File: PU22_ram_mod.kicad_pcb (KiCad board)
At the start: 2 copper layers, 39.2 x 94.7 mm, 11 parts, among them J1 MOBO, J2 BA8, J3 BA10

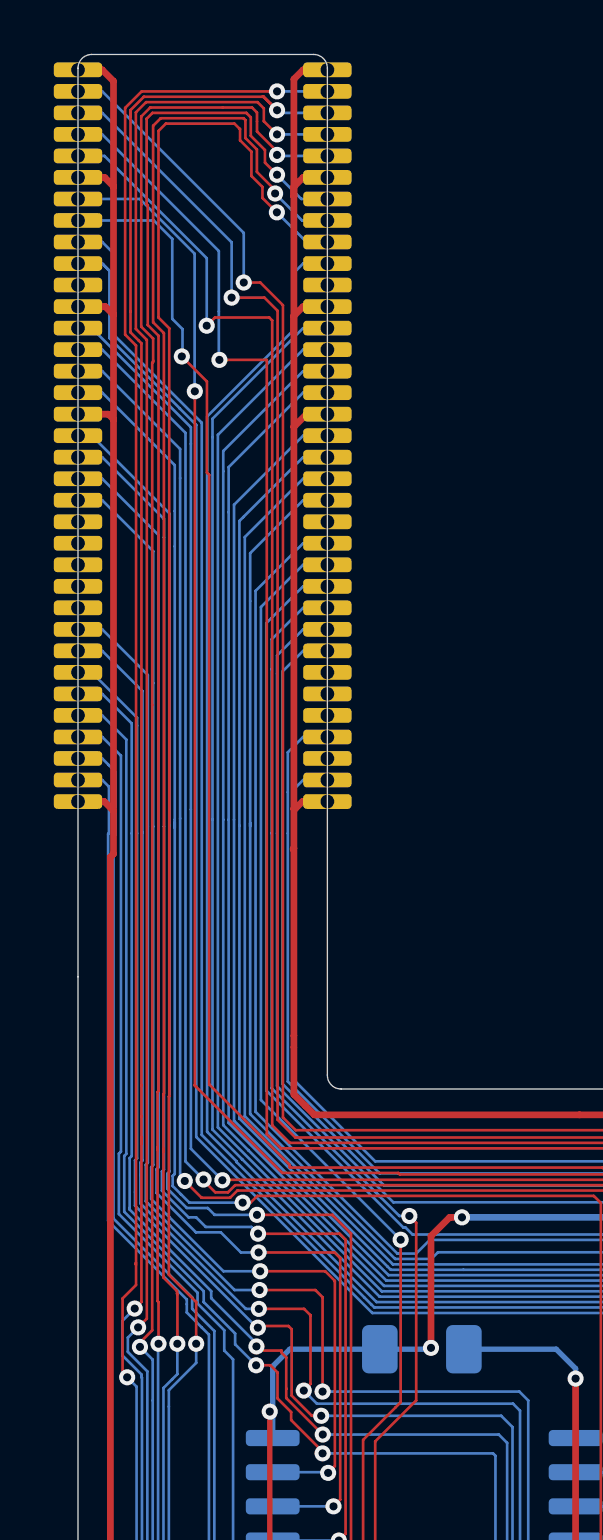
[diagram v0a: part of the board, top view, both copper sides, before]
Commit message: Tweaked traces a bit
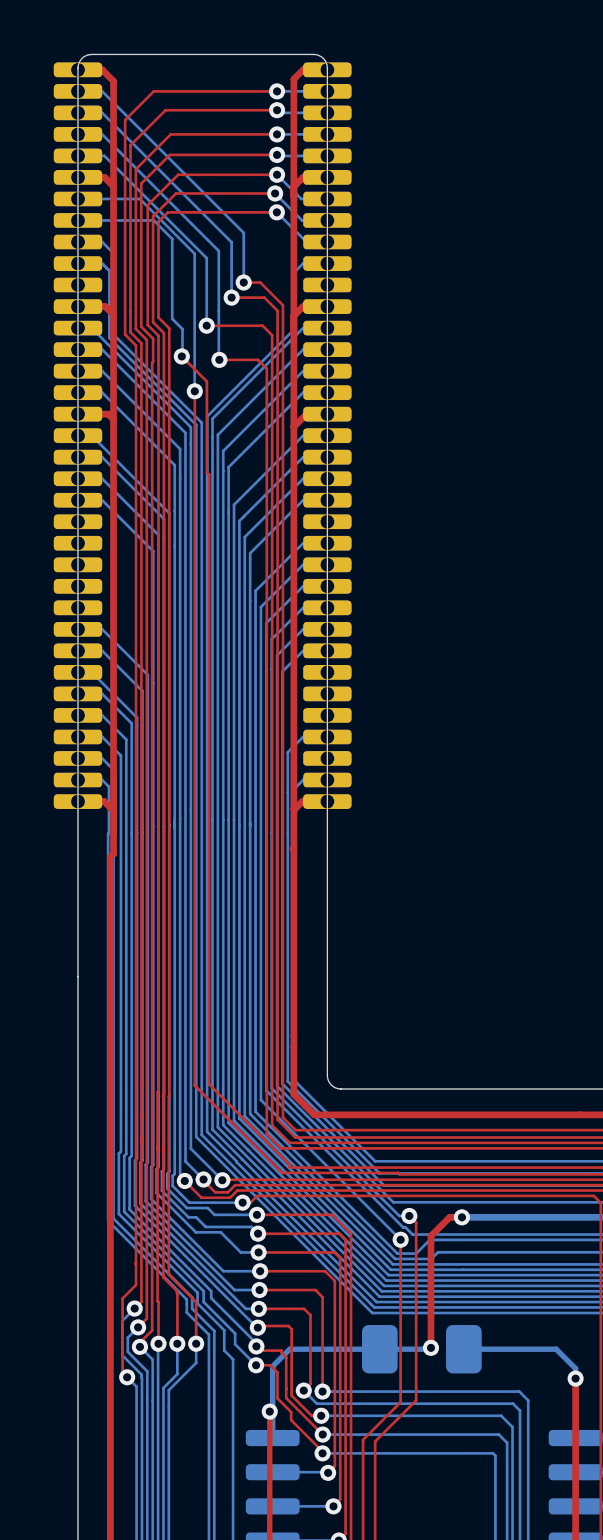
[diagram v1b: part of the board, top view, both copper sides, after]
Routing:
- net /D25: track 96.8 -> 91.1 mm
- net /D26: track 97.5 -> 92.2 mm
- net /D27: track 98.2 -> 93.7 mm
- net /D28: track 93.0 -> 89.6 mm
- net /D29: track 92.0 -> 89.5 mm
- net /D30: track 91.3 -> 89.4 mm
- net /D3: track 94.5 -> 94.0 mm
